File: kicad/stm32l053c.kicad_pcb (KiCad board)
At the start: 2 copper layers, 52 x 35 mm, 41 parts, among them P1 SWD, P2 PWR, Q1 Q_PNP_BEC, SW1 SW_PUSH, SW2 SW_PUSH, SW3 SW_PUSH, U1 STM32L053C8_LQFP48, U2 TLV61225, U3 um66t, Y1 Crystal

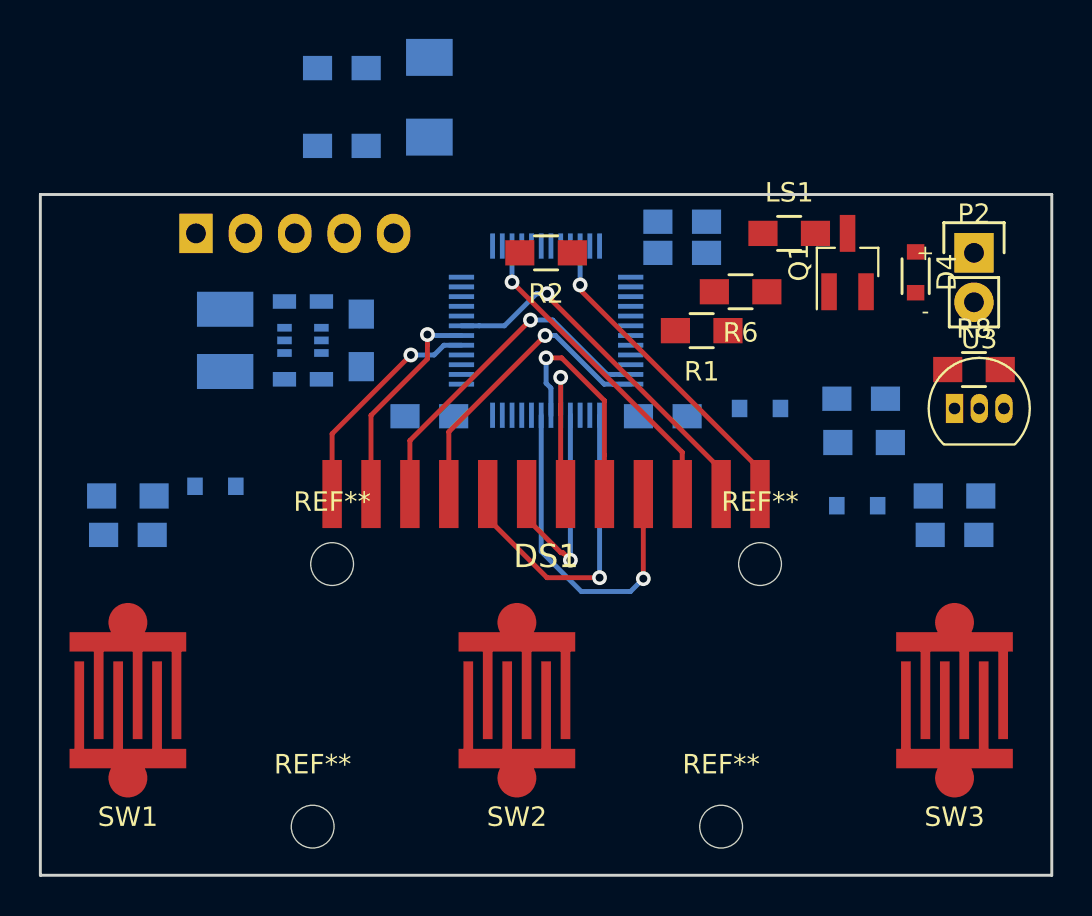
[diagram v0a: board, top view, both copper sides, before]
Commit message: PNP & more layout
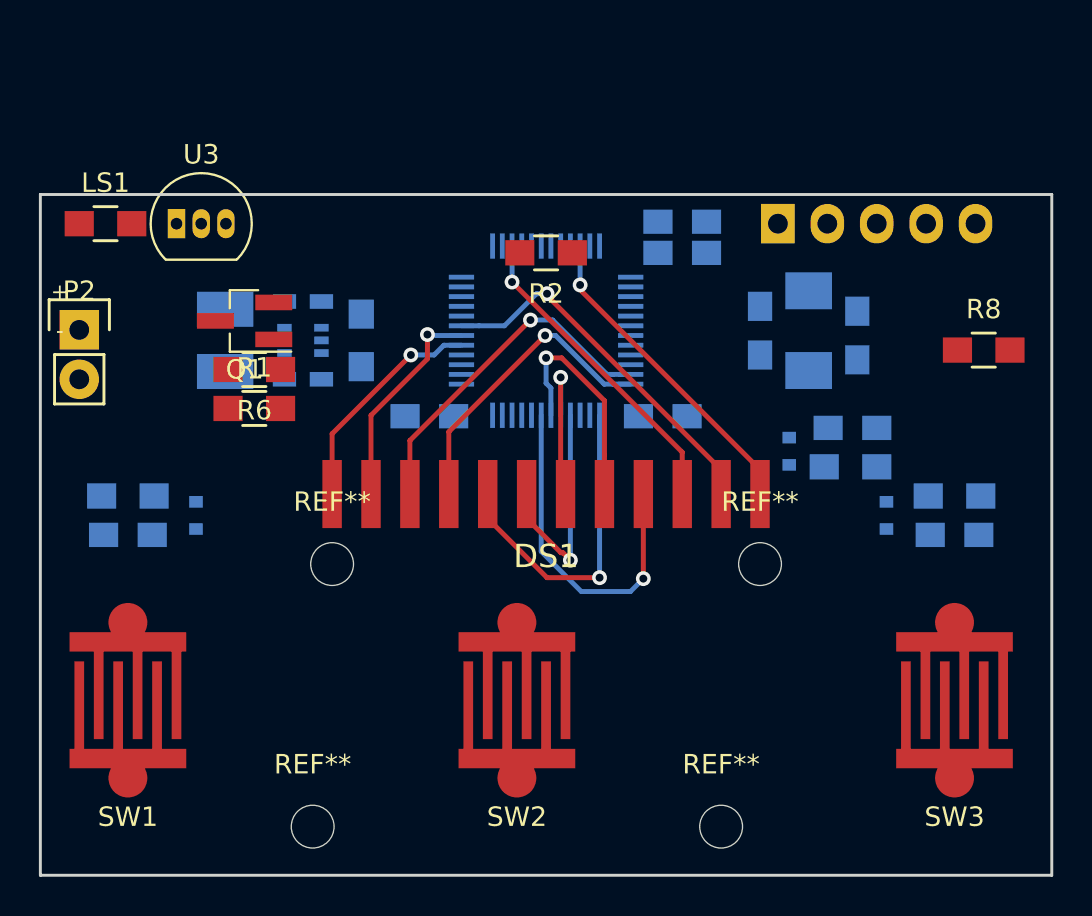
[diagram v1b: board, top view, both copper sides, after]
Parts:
- removed D4: D, Diodes_SMD:D_0805
- D1, D2, D3: footprint Diodes_SMD:D_0805 -> Diodes_SMD:SOD-523
- Q1: value Q_PNP_BEC -> BC807
- R8: value 1K -> 0
- U2: footprint TO_SOT_Packages_SMD:SC-70-6 -> theapi:SC-70-6
- moved P2 46.2 mm to (119.0, 92.6)
- moved U3 41.1 mm to (124.0, 87.1)
- moved LS1 35.2 mm to (120.3, 87.1)
- moved Q1 31.1 mm to (127.5, 92.1), turned to 180 degrees
- moved P1 29.9 mm to (154.9, 87.1)
- moved C7 29.9 mm to (159.0, 92.8), turned to 270 degrees
- moved R6 25.3 mm to (128.0, 94.6)
- moved C6 23.5 mm to (154.0, 92.6), turned to 90 degrees
- moved R1 23.3 mm to (128.0, 96.6), turned to 0 degrees
- moved Y1 22.9 mm to (156.5, 92.6)
- moved D2 2.66 mm to (155.5, 98.8), turned to 270 degrees
- moved D1 1.80 mm to (125.0, 102.1), turned to 270 degrees
- moved D3 1.58 mm to (160.5, 102.1), turned to 270 degrees
- moved C10 1.57 mm to (158.8, 97.6), turned to 0 degrees
- moved R4 1.43 mm to (158.7, 99.6)
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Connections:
- C3 pad 1: VDD -> /VDDA
- LS1 pad 1: +BATT -> Net-(LS1-Pad1)
- LS1 pad 2: Net-(D4-Pad2) -> Earth
- Q1 pad 2: Earth -> +BATT
- Q1 pad 3: Net-(D4-Pad2) -> Net-(LS1-Pad1)
- R8 pad 1: Net-(R8-Pad1) -> /VDDA
- R8 pad 2: /MELODY -> VDD
- U1 pad 9: VDD -> /VDDA
- U3 pad 2: Net-(R8-Pad1) -> /MELODY
